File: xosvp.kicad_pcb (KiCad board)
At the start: 2 copper layers, 49.5 x 50 mm, 14 parts

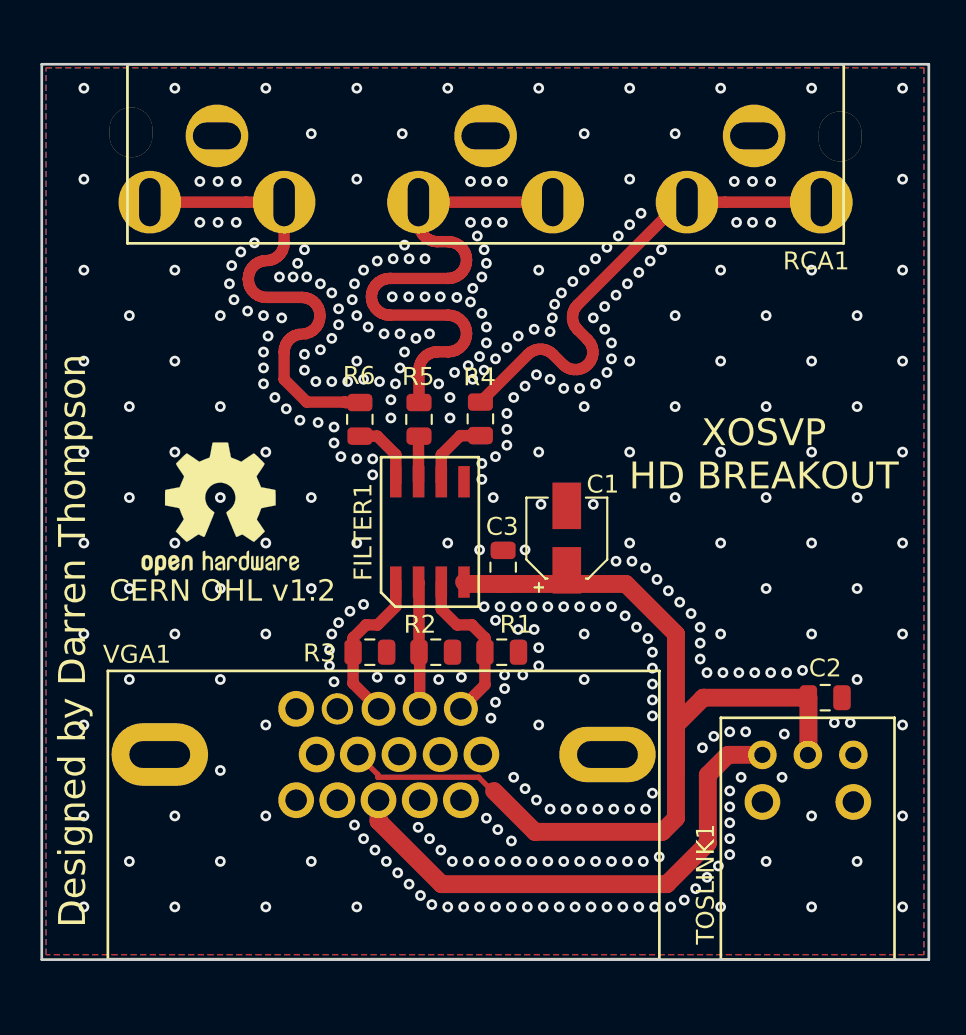
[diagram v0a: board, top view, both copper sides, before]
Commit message: Initial Commit. Major redesign, yet to be finished.
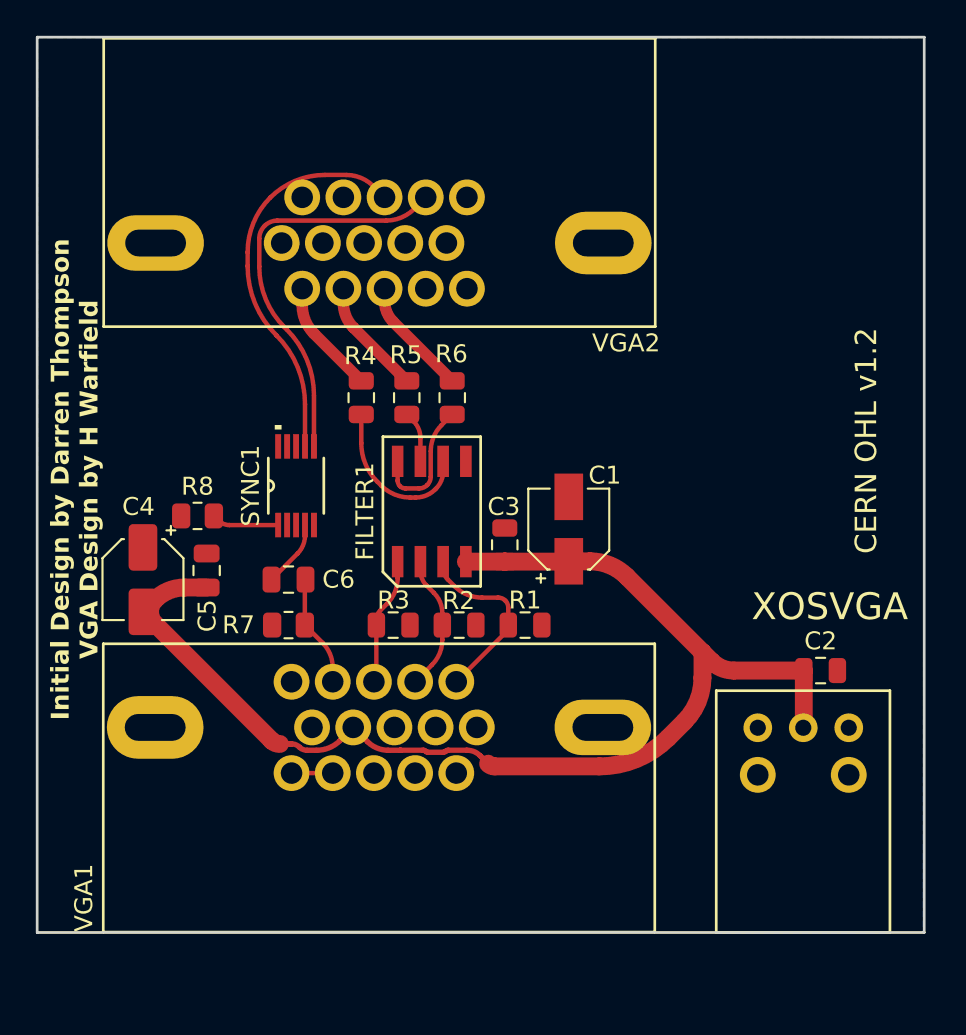
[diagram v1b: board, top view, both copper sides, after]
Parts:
- removed RCA1: PJRAN3XIU03X, xosvp:PJRAN3X1U
- removed REF**: OSHW-Logo2_9.8x8mm_SilkScreen, Symbol:OSHW-Logo2_9.8x8mm_SilkScreen
- added C4: 10uF, Capacitor_SMD:CP_Elec_4x5.8, F.Cu at (26.2, 52.8)
- added C5: 0.1uF, Capacitor_SMD:C_0805_2012Metric, F.Cu at (29.7, 52.3)
- added C6: 0.1uF, Capacitor_SMD:C_0805_2012Metric, F.Cu at (34.3, 52.8)
- added R7: R75, Resistor_SMD:R_0805_2012Metric, F.Cu at (34.3, 55.4)
- added R8: 10K, Resistor_SMD:R_0805_2012Metric, F.Cu at (29.2, 49.3)
- added SYNC1: LMH1980, xosvp:LMH1980, F.Cu at (34.7, 47.6)
- added VGA2: DB15_Female_HighDensity_MountingHoles, xosvp:AHDF15A, F.Cu at (39.4, 34.0)
- moved R4 6.76 mm to (38.4, 42.7)
- moved R6 5.30 mm to (43.4, 42.7)
- moved R1 2.00 mm to (47.5, 55.4)
- moved R2 2.00 mm to (43.8, 55.4)
- moved R3 2.00 mm to (40.1, 55.4)
- moved C2 1.54 mm to (64.0, 57.9)
- moved TOSLINK1 1.54 mm to (63.0, 65.8)
- moved VGA1 1.54 mm to (39.3, 61.1)
- moved R5 1.39 mm to (40.9, 42.7)
- moved C3 1.25 mm to (46.4, 50.9)
- moved FILTER1 1.15 mm to (42.3, 49.0)
- moved C1 0.51 mm to (49.9, 50.0)
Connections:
- net PB_BLUE renamed BLUE
- net PR_RED renamed RED
- net Y_GREEN renamed GREEN
- C1 pad 2: Earth -> GND
- C2 pad 2: Earth -> GND
- C3 pad 2: Earth -> GND
- FILTER1 pad 5: Earth -> GND
- R1 pad 2: Earth -> GND
- R2 pad 2: Earth -> GND
- R3 pad 2: Earth -> GND
- TOSLINK1 pad 1: Earth -> GND
- TOSLINK1 pad 4: Earth -> unconnected-(TOSLINK1-Mount-Pad4)
- TOSLINK1 pad 5: Earth -> unconnected-(TOSLINK1-Mount-Pad5)
- VGA1 pad 0: Earth -> GND
- VGA1 pad 10: Earth -> GND
- VGA1 pad 11: Earth -> GND
- VGA1 pad 12: Earth -> GND
- VGA1 pad 14: Earth -> SW1
- VGA1 pad 15: Earth -> SW1
- VGA1 pad 4: Earth -> SYNC
- VGA1 pad 5: Earth -> GND
- VGA1 pad 6: Earth -> GND
- VGA1 pad 7: Earth -> GND
- VGA1 pad 8: Earth -> GND
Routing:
- net SPDIF: track 29.3 -> 0.00 mm
- net Net-(R5-Pad2): track 31.1 -> 6.52 mm
- net H_SYNC: track 0.00 -> 22.7 mm
- net V_SYNC: track 0.00 -> 22.1 mm
- net Net-(R4-Pad2): track 27.5 -> 6.41 mm
- net Net-(R6-Pad2): track 27.6 -> 6.63 mm
- net +5V: track 57.2 -> 67.4 mm
- net SYNC: track 0.00 -> 6.27 mm
- net Net-(FILTER1-OUT1): track 4.14 -> 9.27 mm
- net Net-(SYNC1-REXT): track 0.00 -> 3.76 mm
- net Net-(SYNC1-VIN): track 0.00 -> 3.75 mm
- net Net-(FILTER1-OUT3): track 3.95 -> 7.41 mm
- net SW1: track 0.00 -> 2.30 mm
- net BLUE: track 9.04 -> 7.11 mm
- net RED: track 9.14 -> 10.4 mm
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- added copper zone on B.Cu, net GND
- removed copper zone on B.Cu, net Earth
- removed copper zone on F.Cu, net Earth
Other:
- net class 75ohm removed
- net class Default removed
- net class med removed
- board text added: "Initial Design by Darren Thompson VGA Design by H Warfield"
- board text added: "XOSVGA"
- board text added: "{ "ViaStitching": "0.2", "stitch_zone_0": { "HSpacing": "1", "VSpacing": "1", "Clearance": "0", "Randomize": false } }"
- board text added: "{ "ViaStitching": "0.2", "stitch_zone_0": { "HSpacing": "1", "VSpacing": "1", "Clearance": "0", "Randomize": true } }"
- board text added: "{ "ViaStitching": "0.2", "stitch_zone_0": { "HSpacing": "1", "VSpacing": "1", "Clearance": "0.2", "Randomize": false } }"
- board text added: "{ "ViaStitching": "0.2", "stitch_zone_0": { "HSpacing": "1", "VSpacing": "1", "Clearance": "1", "Randomize": true } }"
- board text removed: "Designed by Darren Thompson"
- board text removed: "XOSVP HD BREAKOUT"
